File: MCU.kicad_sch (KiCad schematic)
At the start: 31 parts, among them IC1 R7FA4M1AB3CFM#AA0, J7 Conn_01x02_Pin, SW1 SW_MEC_5E, Y1 ABM8W-12.0000MHZ-8-K1Z-T3

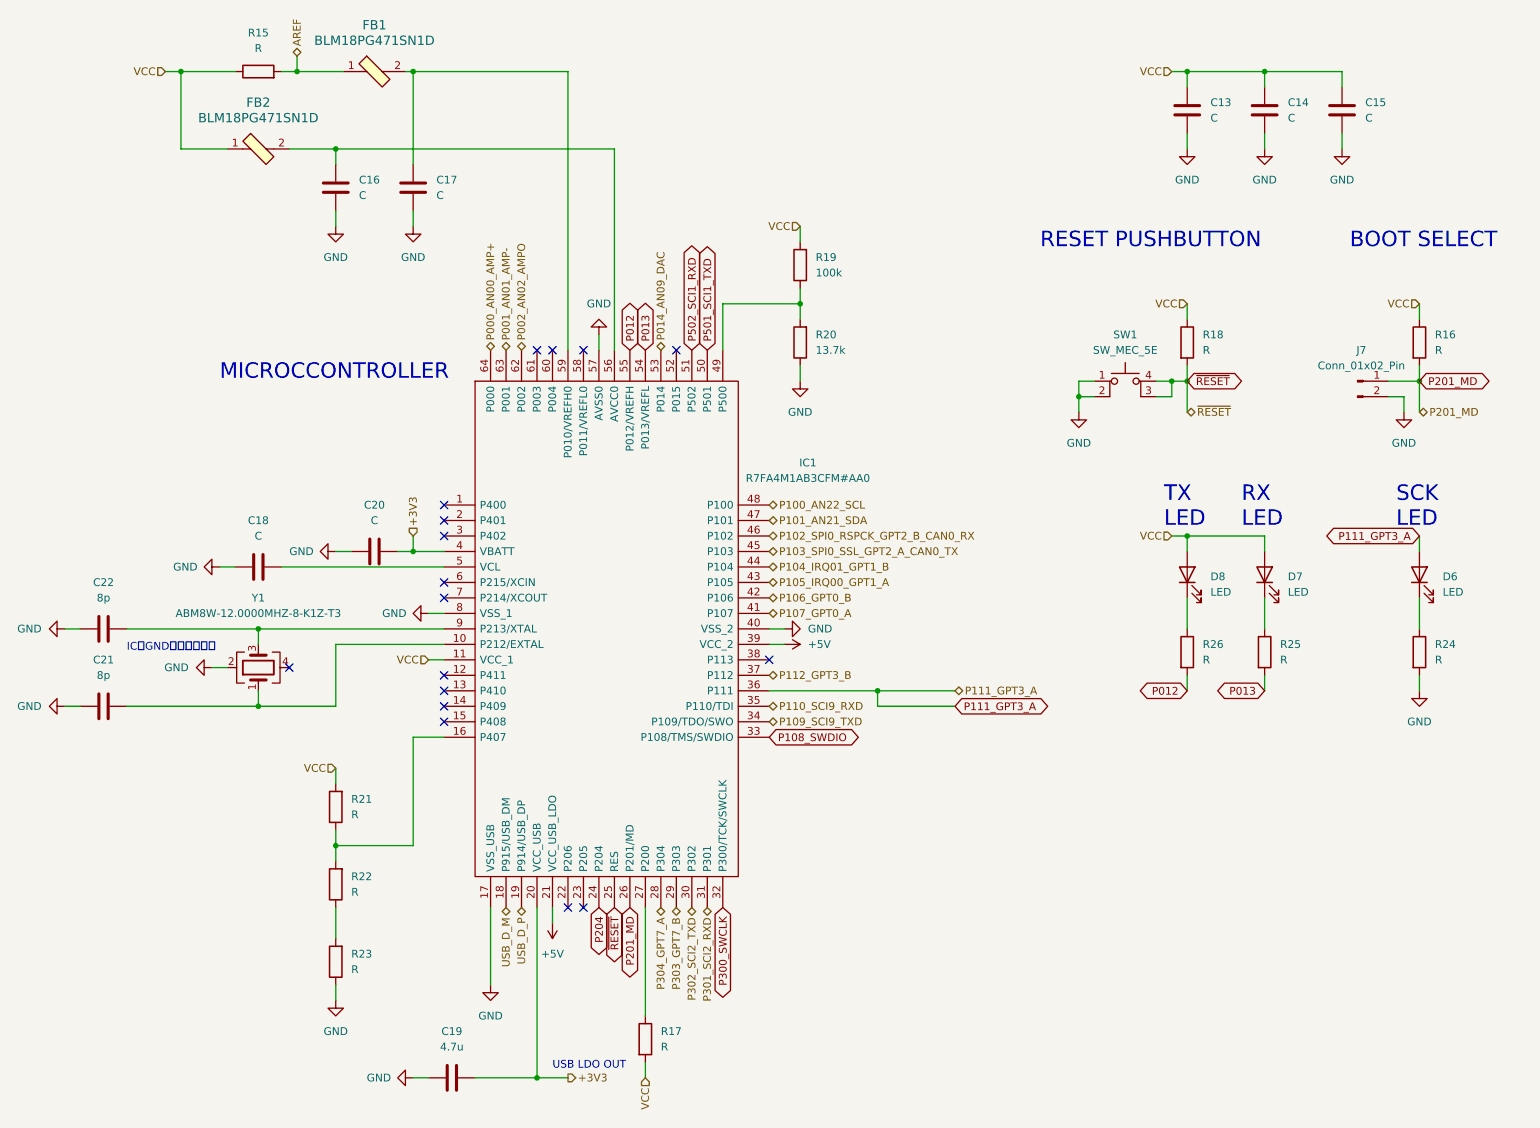
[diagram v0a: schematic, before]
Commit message: modify, add I/O port
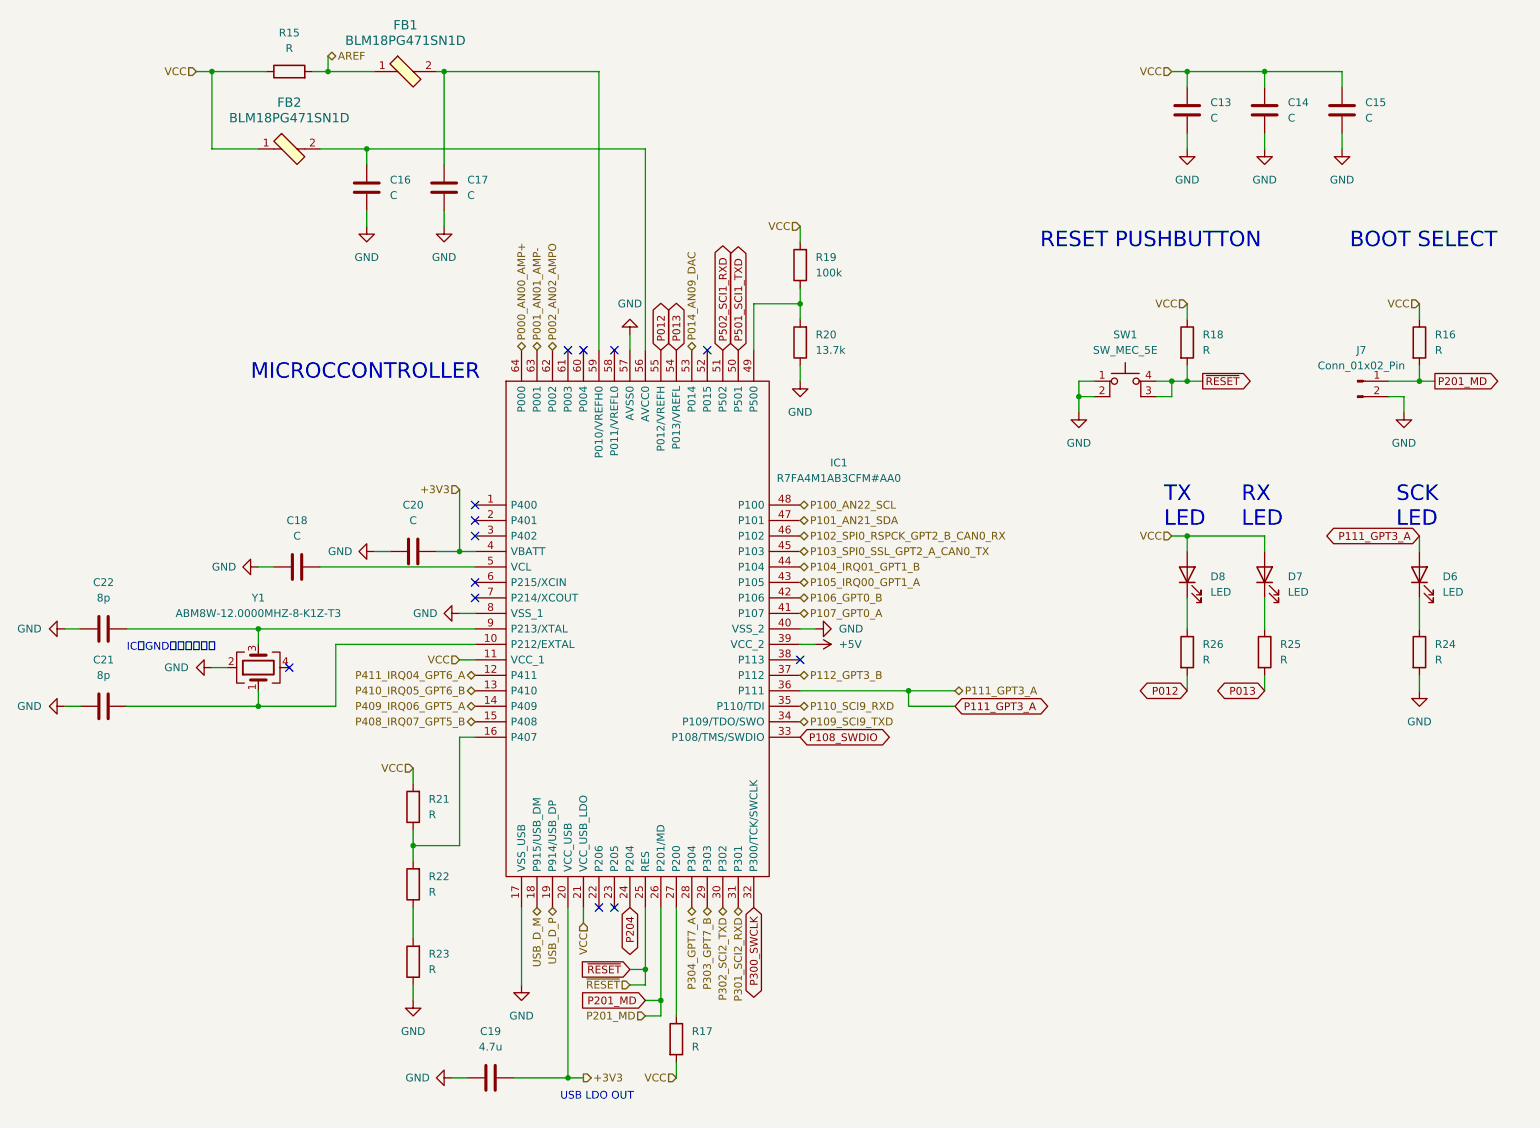
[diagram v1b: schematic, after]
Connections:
- net +5V: no longer IC1.21 (VCC_USB_LDO)
- net VCC: now also IC1.21 (VCC_USB_LDO)
- net P411_IRQ04_GPT6_A: now reaches IC1.12 (P411)
- net P410_IRQ05_GPT6_B: now reaches IC1.13 (P410)
- net P409_IRQ06_GPT5_A: now reaches IC1.14 (P409)
- net P408_IRQ07_GPT5_B: now reaches IC1.15 (P408)
- no-connect marks 17 -> 13
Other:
- moved on the sheet: C16, C17, C18, C19, C20, FB1, FB2, IC1, R15, R17, R21, R22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
